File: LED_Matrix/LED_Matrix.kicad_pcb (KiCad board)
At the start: 2 copper layers, 44.5 x 29.2 mm, 21 parts, among them J1 Conn_01x02, U1 NE555P

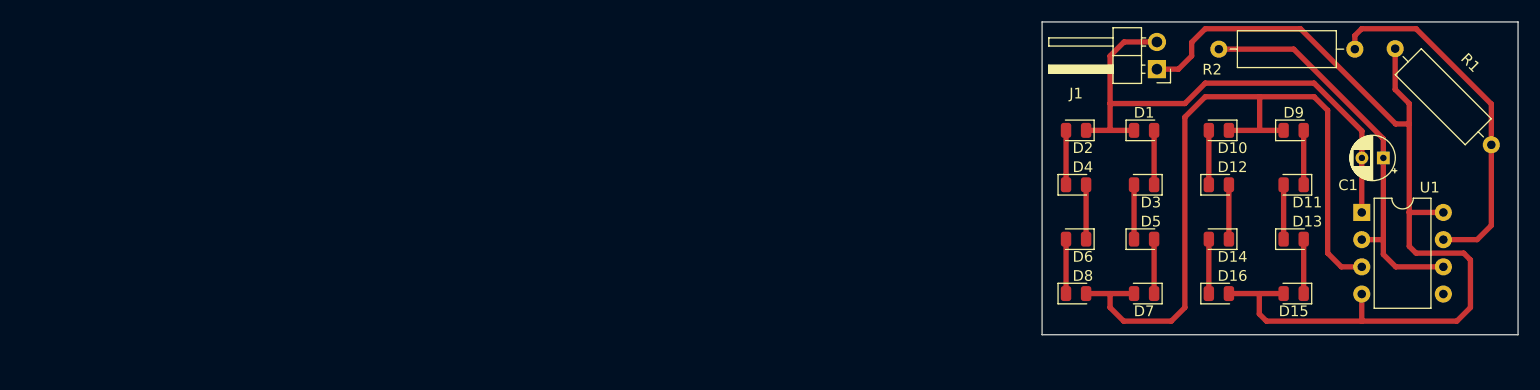
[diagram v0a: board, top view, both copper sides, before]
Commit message: 20230812_1329
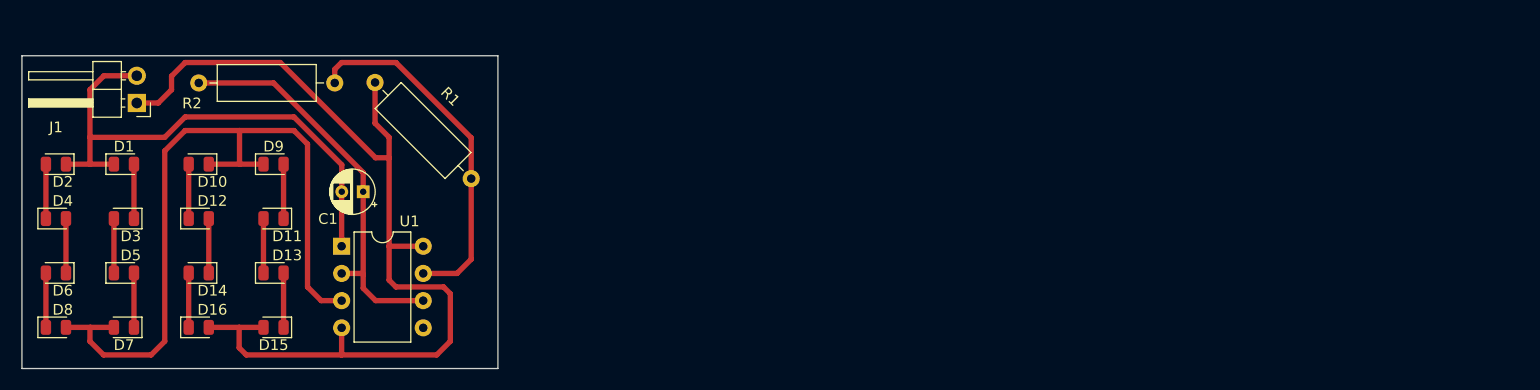
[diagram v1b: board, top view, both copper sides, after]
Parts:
- moved J1 95.3 mm to (38.5, 96.3)
- moved D10 95.3 mm to (44.3, 102.1)
- moved D12 95.3 mm to (44.3, 107.1)
- moved D14 95.3 mm to (44.3, 112.2)
- moved D16 95.3 mm to (44.3, 117.3)
- moved U1 95.3 mm to (57.7, 109.7)
- moved C1 95.3 mm to (59.7, 104.6)
- moved D1 95.3 mm to (37.3, 102.1)
- moved D11 95.3 mm to (51.3, 107.1)
- moved D13 95.3 mm to (51.3, 112.2)
- moved D15 95.3 mm to (51.3, 117.3)
- moved D2 95.3 mm to (31.0, 102.1)
- moved D3 95.3 mm to (37.3, 107.1)
- moved D4 95.3 mm to (31.0, 107.1)
- moved D5 95.3 mm to (37.3, 112.2)
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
